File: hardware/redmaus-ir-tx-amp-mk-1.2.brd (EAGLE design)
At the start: 15.2 x 15.2 mm, 13 parts, among them Q1 MMBT2222A, Q2 MMBT2222A, Q3 MMBT2222A, Q4 MMBT2222A

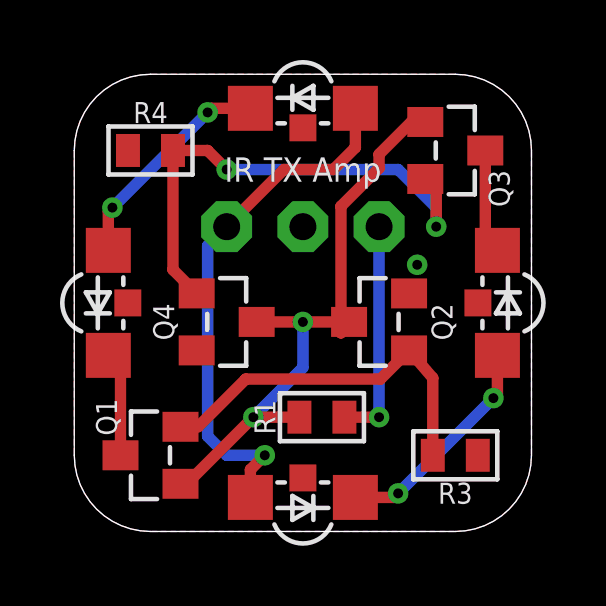
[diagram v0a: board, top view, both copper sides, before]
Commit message: moar boards
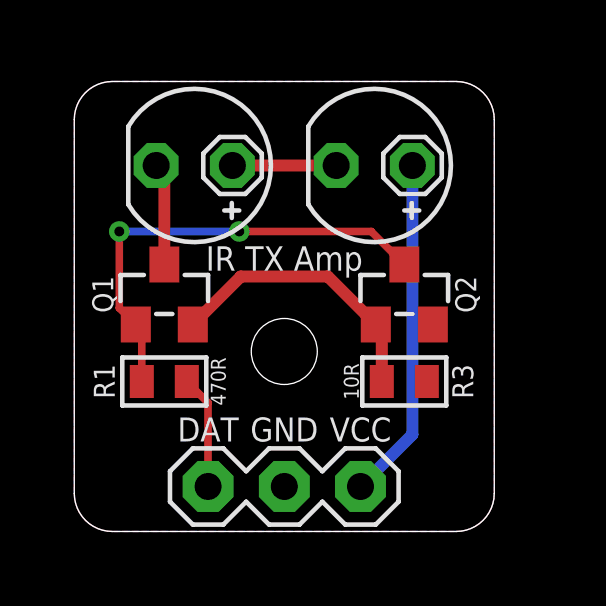
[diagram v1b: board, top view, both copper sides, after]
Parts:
- removed LED3, LED4: LED3MMX2MM-SIDE-SMD, a_parts:LED-3MMX2MM-SIDE-SMD
- removed Q3, Q4: MMBT2222A, a_parts:SOT23
- removed R4: 10R, a_parts:R0603-TIGHTER
- LED1, LED2: value LED3MMX2MM-SIDE-SMD -> LED5MM_SHORTPADS; device a_parts:LED-3MMX2MM-SIDE-SMD -> a_parts:LED5MM_SHORTPADS
- moved JP1 8.68 mm to (7.00, 1.50), flipped to the top
- moved LED1 5.68 mm to (4.00, 12.2)
- moved R1 5.39 mm to (3.00, 5.00)
- moved Q1 5.38 mm to (3.00, 7.90), turned to 0 degrees
- moved LED2 3.38 mm to (10.0, 12.2), turned to 180 degrees
- moved R3 2.99 mm to (11.0, 5.00)
- moved Q2 1.24 mm to (11.0, 7.90), turned to 0 degrees
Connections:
- removed net N$2: LED3.K, Q3.3
- removed net N$5: Q3.2, Q4.1, R4.2
- removed net N$6: LED3.A, LED4.K
- net DATA-AMP: no longer Q3.1, Q4.3
- net GND: no longer Q4.2, R4.1
- net VCC: no longer LED4.A
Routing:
- net N$5: track 17.0 -> 0.00 mm, vias 2 -> 0
- net N$6: track 7.45 -> 0.00 mm, vias 2 -> 0
- net VCC: track 17.7 -> 11.4 mm, vias 1 -> 0
- net DATA-AMP: track 20.8 -> 15.3 mm
- net N$1: track 7.45 -> 3.46 mm, vias 2 -> 0
- net DATA: track 7.50 -> 3.79 mm, vias 1 -> 0
- net N$2: track 3.50 -> 0.00 mm
- net N$4: track 12.5 -> 9.41 mm
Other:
- board size 15.2 x 15.2 mm -> 14 x 15 mm
